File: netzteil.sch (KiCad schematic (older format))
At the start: 14 parts, among them J1 OSTTC022162, J2 Conn_01x02_Male, J3 Conn_01x03_Male, J4 Conn_01x02_Male, Q1 BC847, Q2 BC847

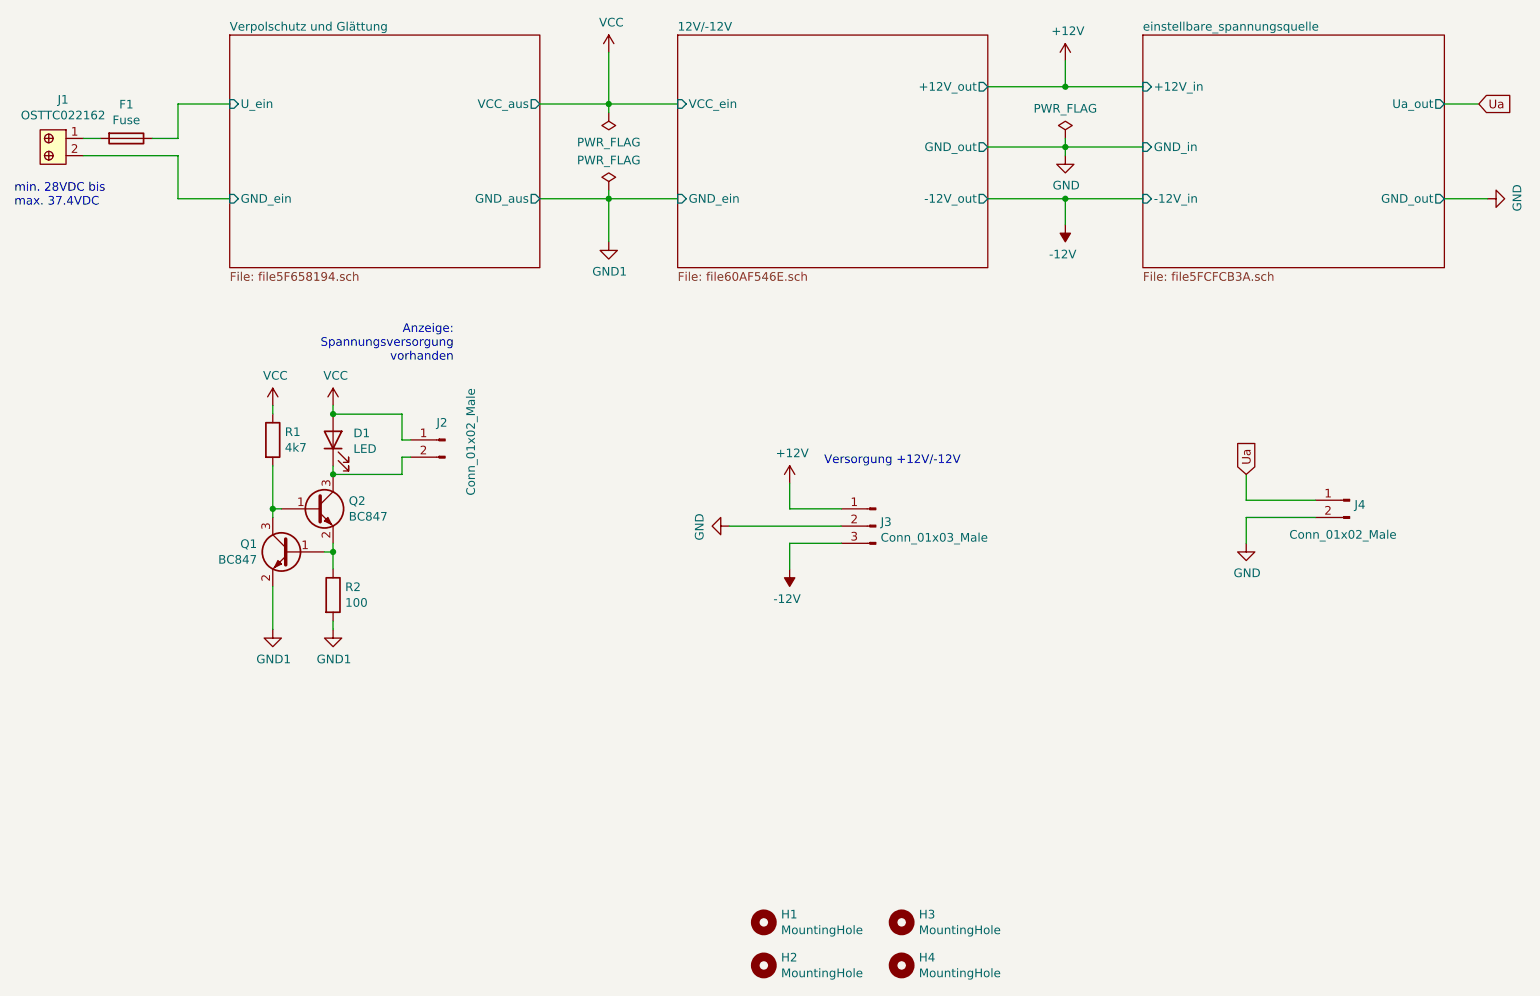
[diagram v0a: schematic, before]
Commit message: pcb netzteil rev. 1.0 finished
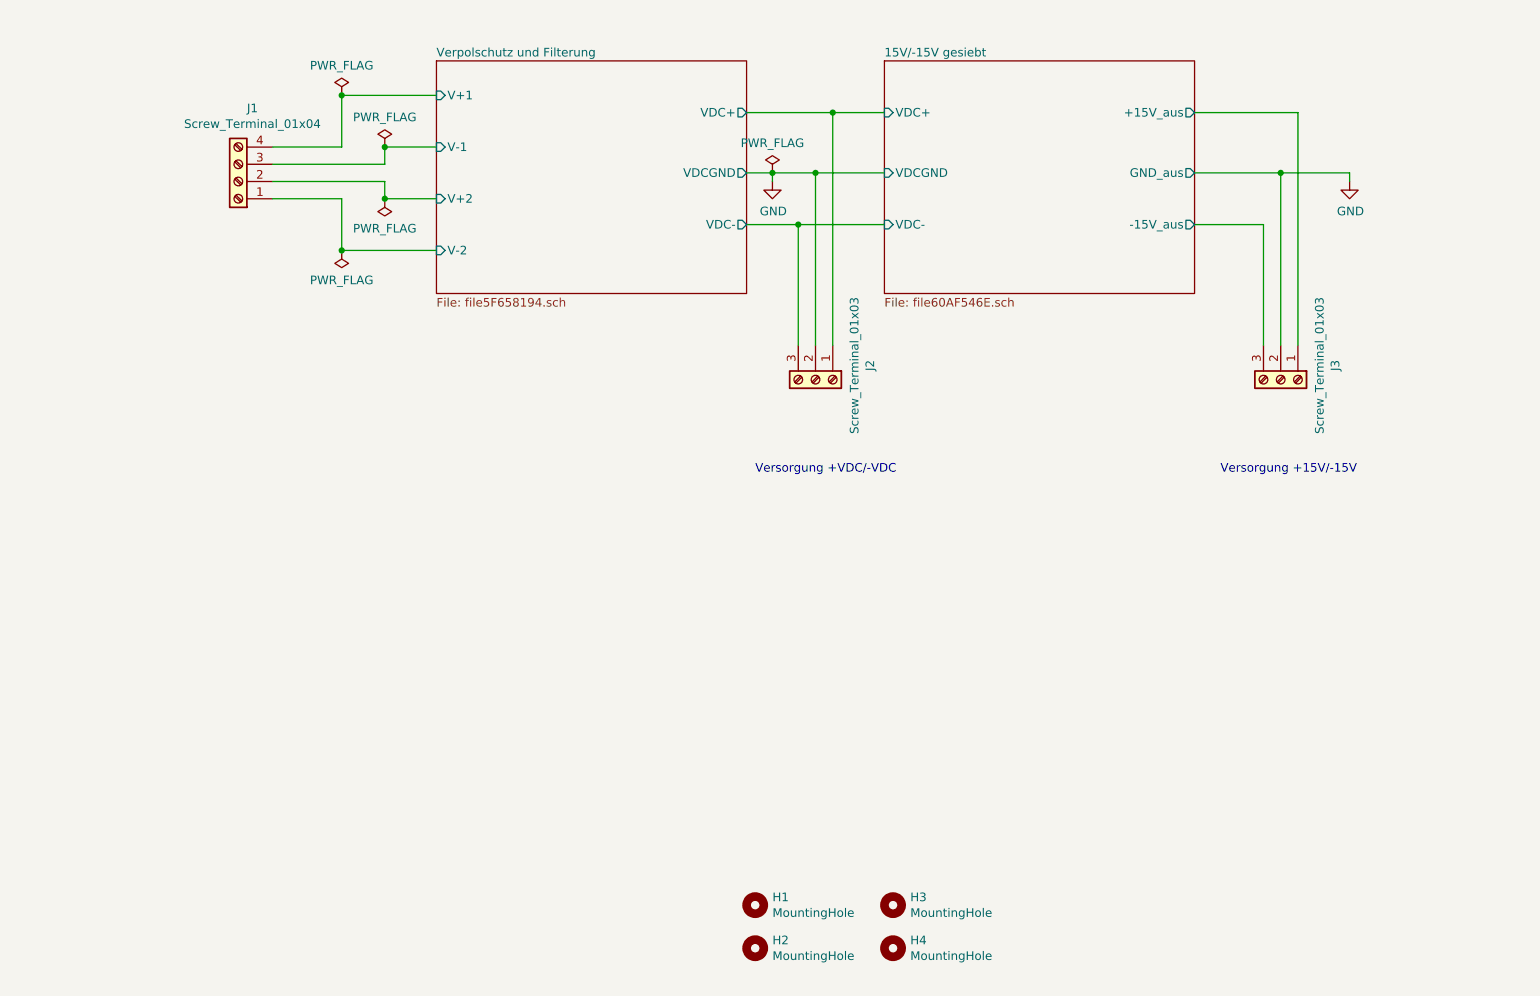
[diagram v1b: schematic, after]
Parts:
- removed D1: LED, LED_SMD:LED_0805_2012Metric_Pad1.15x1.40mm_HandSolder, symbol Device:LED
- removed F1: Fuse, Fuse:Fuseholder_Cylinder-5x20mm_EATON_HBW_Vertical_Closed, symbol Device:Fuse
- removed J1: OSTTC022162, digikey-footprints:Term_Block_1x2_P5.08MM, symbol dk_Terminal-Blocks-Wire-to-Board:OSTTC022162
- removed J2, J4: Conn_01x02_Male, Connector_PinHeader_2.54mm:PinHeader_1x02_P2.54mm_Vertical, symbol Connector:Conn_01x02_Male
- removed J3: Conn_01x03_Male, Connector_PinHeader_2.54mm:PinHeader_1x03_P2.54mm_Vertical, symbol Connector:Conn_01x03_Male
- removed Q1, Q2: BC847, Package_TO_SOT_SMD:SOT-23, symbol Transistor_BJT:BC847
- removed R1: 4k7, Resistor_SMD:R_1206_3216Metric_Pad1.42x1.75mm_HandSolder, symbol Device:R
- removed R2: 100, Resistor_SMD:R_1206_3216Metric_Pad1.42x1.75mm_HandSolder, symbol Device:R
- added J1: Screw_Terminal_01x04, TerminalBlock_Phoenix:TerminalBlock_Phoenix_MKDS-3-4-5.08_1x04_P5.08mm_Horizontal, symbol Connector:Screw_Terminal_01x04
- added J2, J3: Screw_Terminal_01x03, TerminalBlock:TerminalBlock_bornier-3_P5.08mm, symbol Connector:Screw_Terminal_01x03
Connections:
- net GND: now also J2.2 (Pin_2), J3.2 (Pin_2)
- new net 15V/-15V gesiebt/+15V_aus: J3.1 (Pin_1)
- new net 15V/-15V gesiebt/-15V_aus: J3.3 (Pin_3)
- new net 15V/-15V gesiebt/VDC+: J2.1 (Pin_1)
- new net 15V/-15V gesiebt/VDC-: J2.3 (Pin_3)
- new net Verpolschutz und Filterung/V+1: J1.4 (Pin_4)
- new net Verpolschutz und Filterung/V+2: J1.2 (Pin_2)
- new net Verpolschutz und Filterung/V-1: J1.3 (Pin_3)
- new net Verpolschutz und Filterung/V-2: J1.1 (Pin_1)
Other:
- note added: "Versorgung +15V/-15V"
- note added: "Versorgung +VDC/-VDC"
- note removed: "Anzeige: \nSpannungsversorgung\nvorhanden"
- note removed: "Versorgung +12V/-12V"
- note removed: "min. 28VDC bis \nmax. 37.4VDC"
- moved on the sheet: H1, H2, H3, H4
